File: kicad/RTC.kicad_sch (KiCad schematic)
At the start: 14 parts, among them J5 Conn_01x02_Pin, Q6 PMOS, U6 PCF8523T, Y1 ABS07AIG-32.768KHZ-7-T

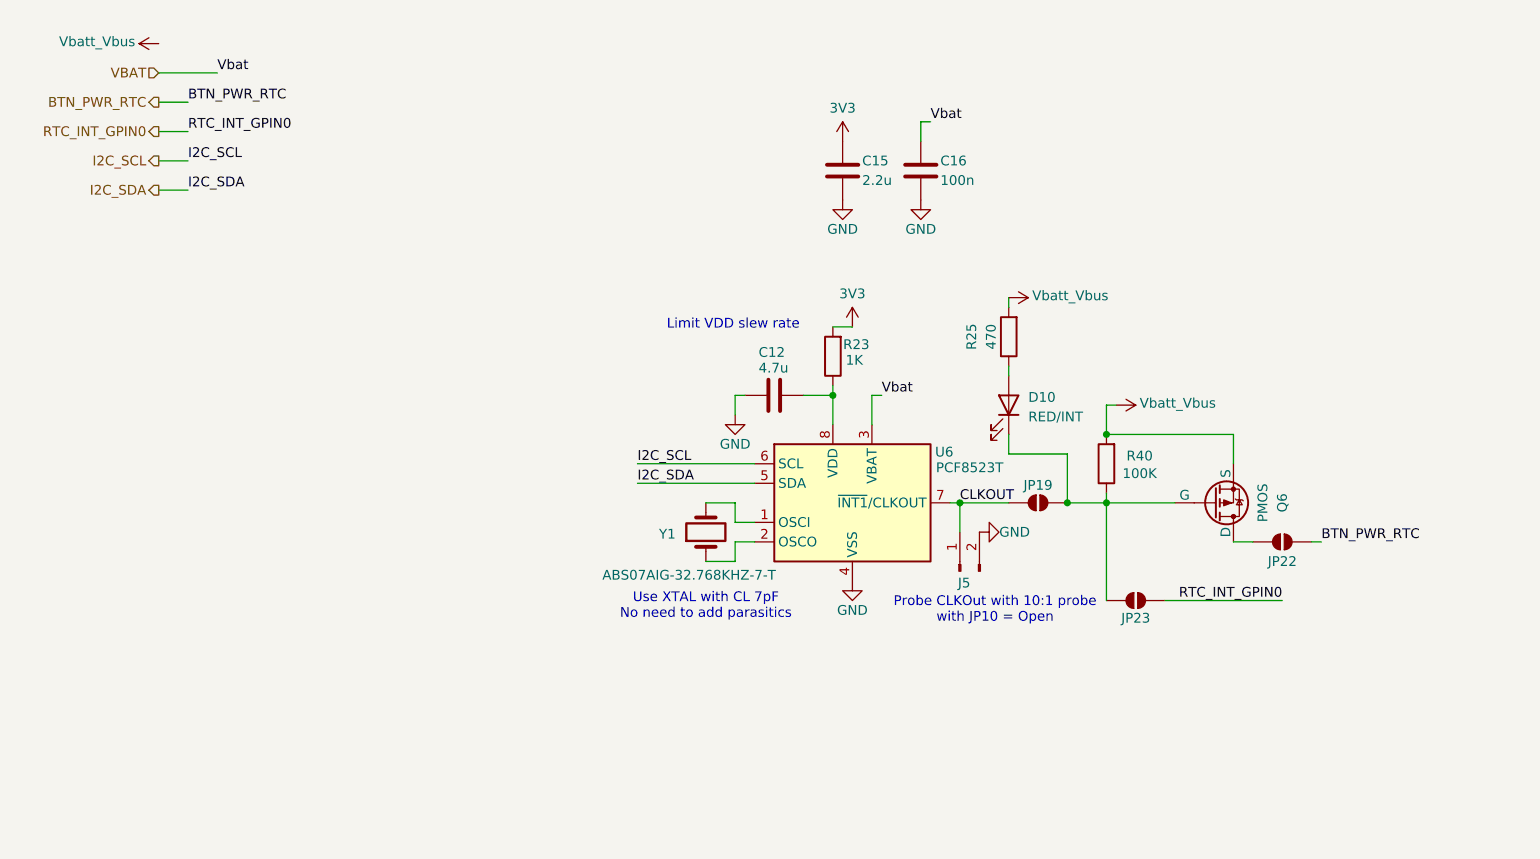
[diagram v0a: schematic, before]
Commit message: pre ERC
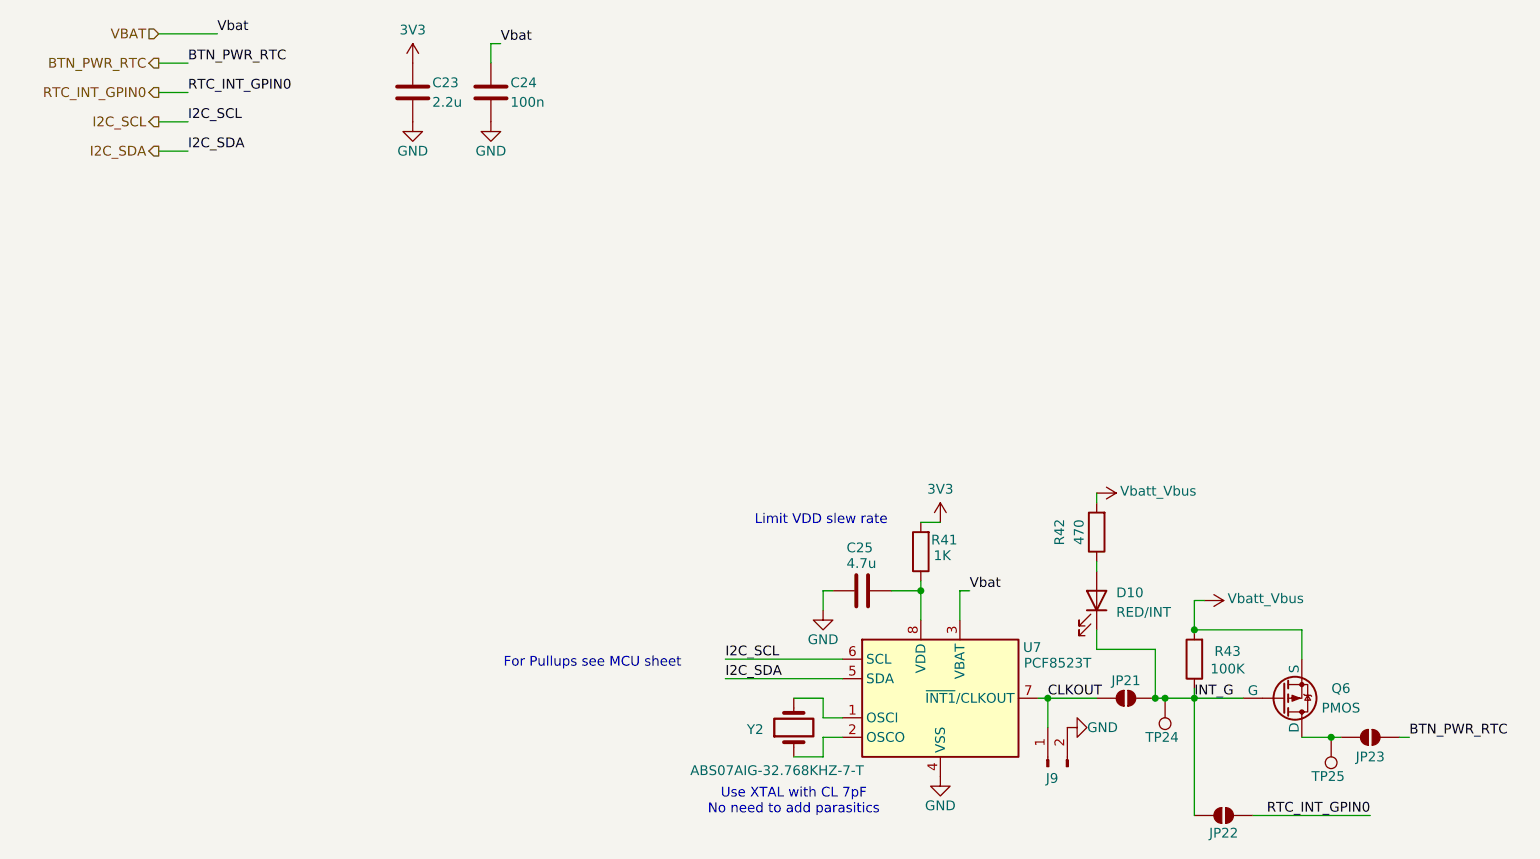
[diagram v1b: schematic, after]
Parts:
- added TP24: INT_G, project footprints:TestPoint_THTPad_D2.0mm_Drill1.0mm, symbol Connector:TestPoint
- added TP25: INT_D, project footprints:TestPoint_THTPad_D2.0mm_Drill1.0mm, symbol Connector:TestPoint
- C23: renamed from C15; footprint (none) -> Capacitor_SMD:C_0805_2012Metric_Pad1.18x1.45mm_HandSolder; MPN (none) -> (Generic); Manufacturer (none) -> (Generic); Package (none) -> 0805; Subsystem (none) -> 07-RTC; Supplier 1 (none) -> (Generic)
- C24: renamed from C16; footprint (none) -> Capacitor_SMD:C_0805_2012Metric_Pad1.18x1.45mm_HandSolder; MPN (none) -> (Generic); Manufacturer (none) -> (Generic); Package (none) -> 0805; Subsystem (none) -> 07-RTC; Supplier 1 (none) -> (Generic)
- C25: renamed from C12; footprint (none) -> Capacitor_SMD:C_0805_2012Metric_Pad1.18x1.45mm_HandSolder; MPN (none) -> (Generic); Manufacturer (none) -> (Generic); Package (none) -> 0805; Subsystem (none) -> 07-RTC; Supplier 1 (none) -> (Generic)
- D10: Subsystem 06-MCU-IO -> 07-RTC
- J9: renamed from J5; footprint (none) -> Connector_PinHeader_2.54mm:PinHeader_1x02_P2.54mm_Vertical; Subsystem (none) -> 07-RTC
- JP21: renamed from JP19; Subsystem (none) -> 07-RTC
- JP22: renamed from JP23; Subsystem (none) -> 07-RTC
- JP23: renamed from JP22; Subsystem (none) -> 07-RTC
- Q6: Subsystem 01-Power-Mux -> 07-RTC
- R41: renamed from R23; Manufacturer (none) -> (Generic); Package (none) -> 0805; Subsystem (none) -> 07-RTC; Supplier 1 (none) -> (Generic)
- R42: renamed from R25; Manufacturer (none) -> (Generic); Subsystem 06-MCU-IO -> 07-RTC; Supplier 1 (none) -> (Generic)
- R43: renamed from R40; Manufacturer (none) -> (Generic); Package (none) -> 0805; Subsystem (none) -> 07-RTC; Supplier 1 (none) -> (Generic)
- U7: renamed from U6; MPN (none) -> PCF8523T/1,118; Manufacturer (none) -> NXP; Package (none) -> SOP-8; Subsystem (none) -> 07-RTC; Supplier 1 (none) -> LCSC; Supplier 1 SKU (none) -> C2651516; Supplier 1 URL (none) -> https://lcsc.com/product-detail/Real-Time-Clocks_NXP-PCF852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
- Y2: renamed from Y1; footprint (none) -> Crystal:Crystal_SMD_3215-2Pin_3.2x1.5mm; Subsystem (none) -> 07-RTC
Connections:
- net at JP23.1 (A), Q6.1 (D): now also TP25.1
- net INT_G: now reaches D10.1 (K), JP21.2 (B), JP22.2 (B), Q6.2 (G), R43.1
- net INT_G: now also TP24.1
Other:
- note added: "For Pullups see MCU sheet"
- note removed: "Probe CLKOut with 10:1 probe with JP10 = Open"
- moved on the sheet: C23, C24, C25, D10, J9, JP21, JP22, JP23, Q6, R41, R42, R43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
